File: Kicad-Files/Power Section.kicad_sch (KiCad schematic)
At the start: 15 parts, among them U2 TPS61023

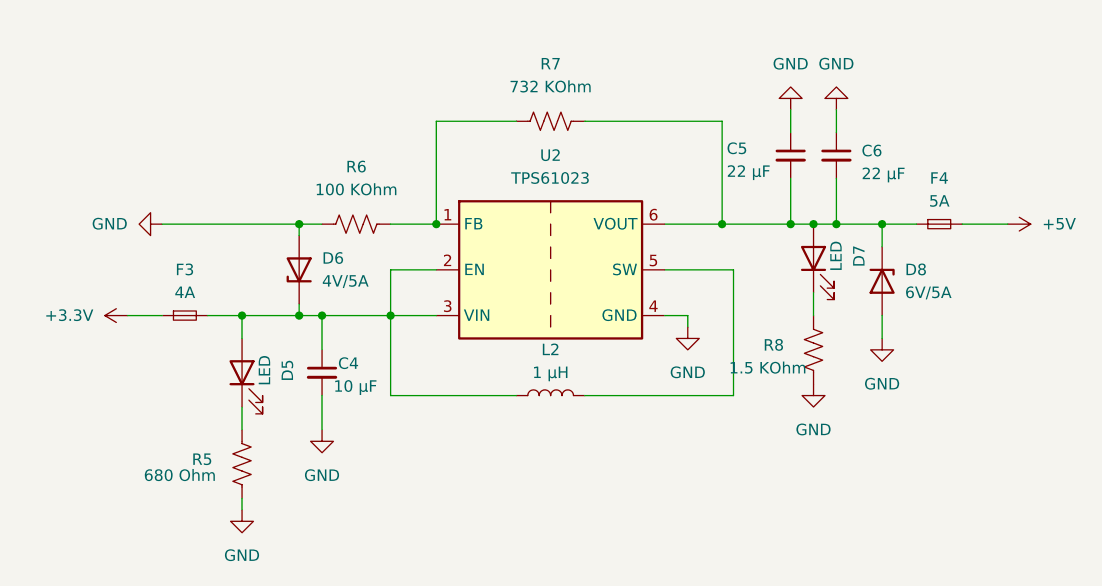
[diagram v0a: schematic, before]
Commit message: Created schematics for 1.1V circuit
Signed-off-by: Jakub Sobota <jakub.sobota@3mdeb.com>
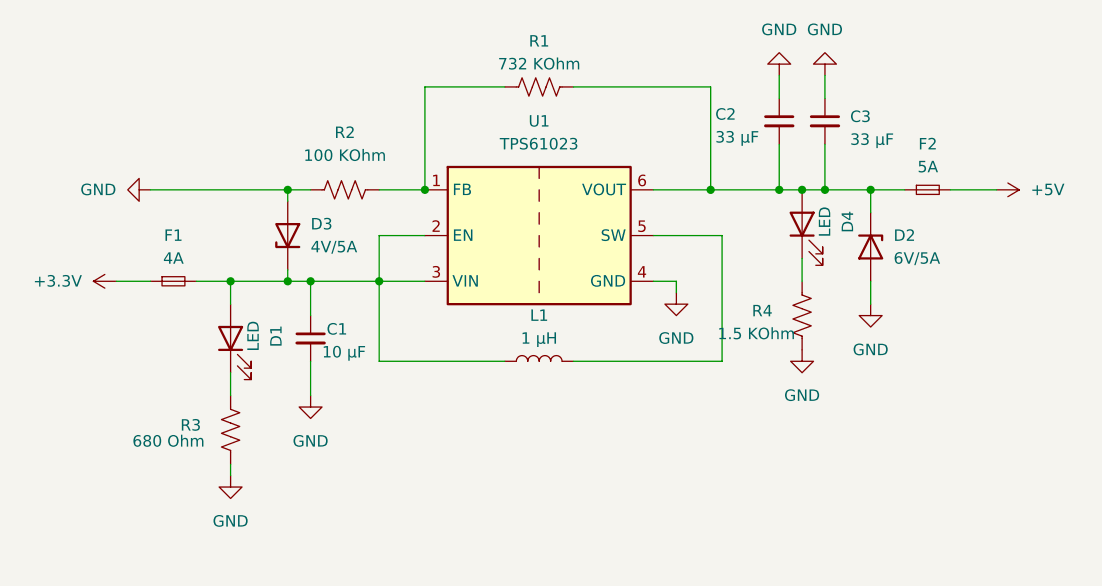
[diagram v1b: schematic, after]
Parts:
- removed C4: 10 μF, Capacitor_SMD:C_0805_2012Metric_Pad1.18x1.45mm_HandSolder, symbol Device:C_Small
- removed C5, C6: 22 μF, Capacitor_SMD:C_1206_3216Metric_Pad1.33x1.80mm_HandSolder, symbol Device:C_Small
- removed D5, D7: LED, LED_SMD:LED_0603_1608Metric_Pad1.05x0.95mm_HandSolder, symbol Device:LED
- removed D6: 4V/5A, Diode_SMD:D_SOD-523, symbol Diode:PTVS5V0Z1USK
- removed D8: 6V/5A, Diode_SMD:D_SOD-523, symbol Diode:PTVS5V0Z1USK
- removed F3: 4A, Fuse:Fuse_0603_1608Metric_Pad1.05x0.95mm_HandSolder, symbol Device:Fuse_Small
- removed F4: 5A, Fuse:Fuse_0603_1608Metric_Pad1.05x0.95mm_HandSolder, symbol Device:Fuse_Small
- removed L2: 1 μH, Inductor_SMD:L_Chilisin_BMRx00050515, symbol Device:L
- removed R5: 680 Ohm, Resistor_SMD:R_0201_0603Metric_Pad0.64x0.40mm_HandSolder, symbol Device:R_US
- removed R6: 100 KOhm, Resistor_SMD:R_0603_1608Metric_Pad0.98x0.95mm_HandSolder, symbol Device:R_US
- removed R7: 732 KOhm, Resistor_SMD:R_0603_1608Metric_Pad0.98x0.95mm_HandSolder, symbol Device:R_US
- removed R8: 1.5 KOhm, Resistor_SMD:R_0201_0603Metric_Pad0.64x0.40mm_HandSolder, symbol Device:R_US
- removed U2: TPS61023, DC-DC_Converter:TPS61023, symbol TPS61023:TPS61023
- added C1: 10 μF, Capacitor_SMD:C_0805_2012Metric_Pad1.18x1.45mm_HandSolder, symbol Device:C_Small
- added C2, C3: 33 μF, Capacitor_SMD:C_0805_2012Metric_Pad1.18x1.45mm_HandSolder, symbol Device:C_Small
- added D1, D4: LED, LED_SMD:LED_0603_1608Metric_Pad1.05x0.95mm_HandSolder, symbol Device:LED
- added D2: 6V/5A, Diode_SMD:D_SOD-523, symbol Diode:PTVS5V0Z1USK
- added D3: 4V/5A, Diode_SMD:D_SOD-523, symbol Diode:PTVS5V0Z1USK
- added F1: 4A, Fuse:Fuse_0603_1608Metric_Pad1.05x0.95mm_HandSolder, symbol Device:Fuse_Small
- added F2: 5A, Fuse:Fuse_0603_1608Metric_Pad1.05x0.95mm_HandSolder, symbol Device:Fuse_Small
- added L1: 1 μH, Inductor_SMD:L_Chilisin_BMRx00050515, symbol Device:L
- added R1: 732 KOhm, Resistor_SMD:R_0603_1608Metric_Pad0.98x0.95mm_HandSolder, symbol Device:R_US
- added R2: 100 KOhm, Resistor_SMD:R_0603_1608Metric_Pad0.98x0.95mm_HandSolder, symbol Device:R_US
- added R3: 680 Ohm, Resistor_SMD:R_0402_1005Metric_Pad0.72x0.64mm_HandSolder, symbol Device:R_US
- added R4: 1.5 KOhm, Resistor_SMD:R_0402_1005Metric_Pad0.72x0.64mm_HandSolder, symbol Device:R_US
- added U1: TPS61023, DC-DC_Converter:TPS61023, symbol TPS61023:TPS61023
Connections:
- net +3.3V: now also F1.1
- net +5V: now also F2.2
- net GND: now also C1.2, C2.1, C3.1, D2.2 (A), D3.2 (A), R2.1, R3.2, R4.2, U1.4 (GND)
- new net: C1.1, D1.2 (A), D3.1 (K), F1.2, L1.1, U1.2 (EN), U1.3 (VIN)
- new net: L1.2, U1.5 (SW)
- new net: D4.1 (K), R4.1
- new net: D1.1 (K), R3.1
- new net: R1.1, R2.2, U1.1 (FB)
- new net: C2.2, C3.2, D2.1 (K), D4.2 (A), F2.1, R1.2, U1.6 (VOUT)
